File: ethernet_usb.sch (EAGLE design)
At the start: 7 parts, among them IC1 LAN9512, X1 MINI-USB_SHIELD4P-85-32004-10X

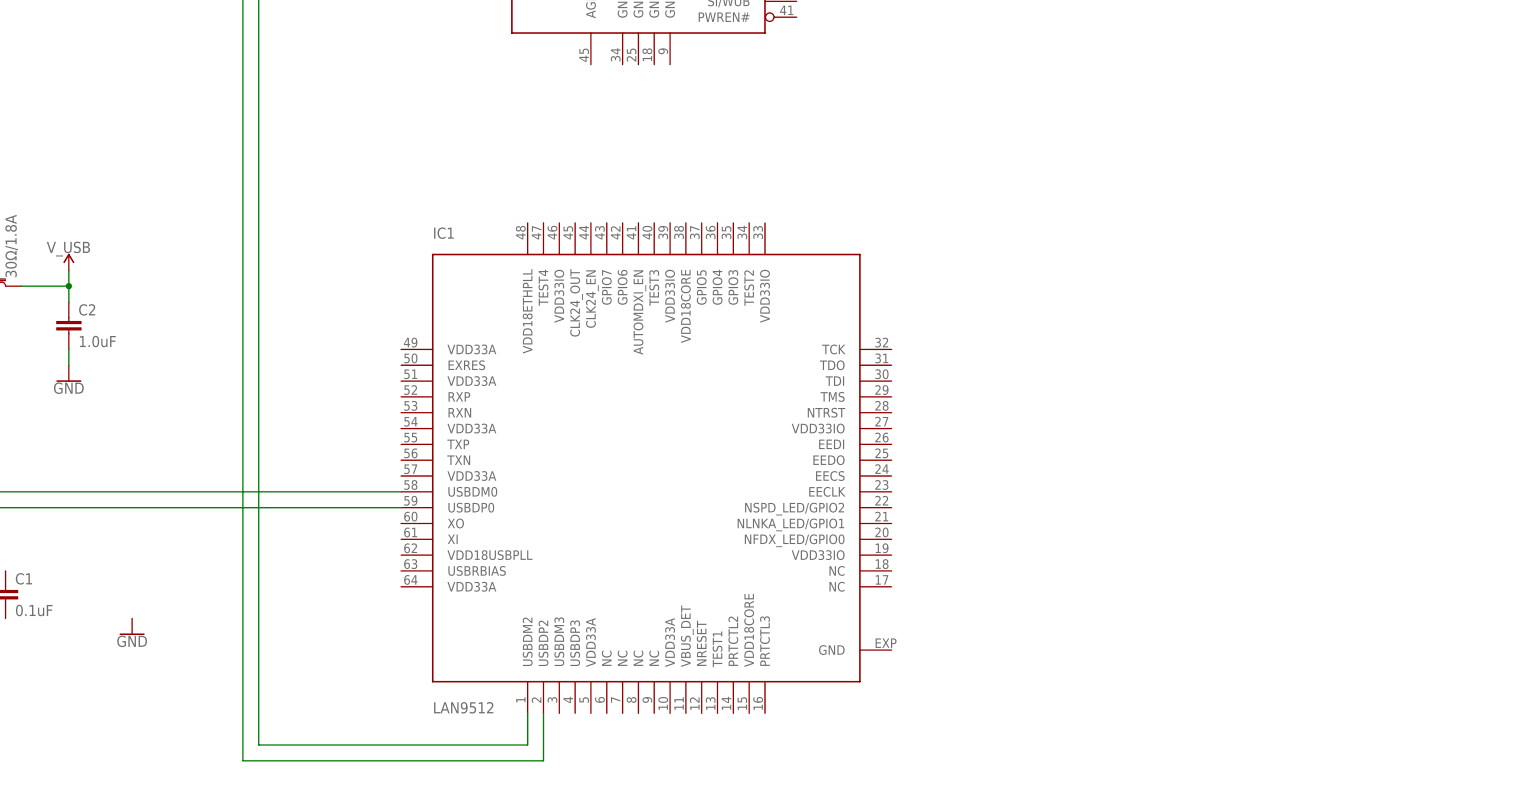
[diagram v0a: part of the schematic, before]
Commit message: snapshot
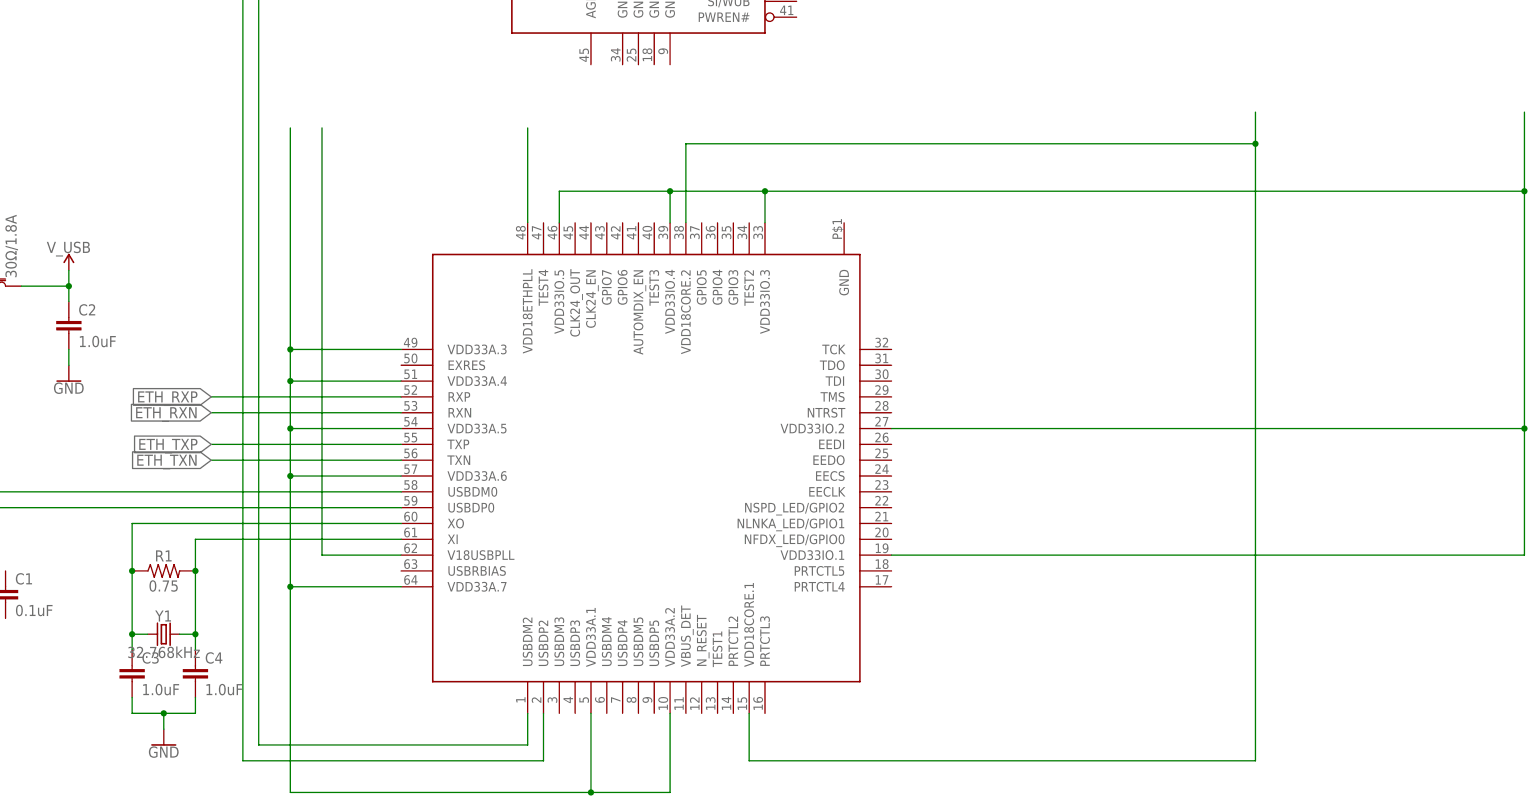
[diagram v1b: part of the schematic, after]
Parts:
- removed IC1: LAN9512, raspberrypi_cm:LAN9512
- added C3, C4: 1.0uF, SparkFun-Capacitors:1.0UF-0805-25V-10%
- added R1: 0.75, SparkFun-Resistors:0.75OHM-0805-1/4W-1%
- added U$2: LAN9514, Eagle-Library:LAN9514
- added Y1: 32.768kHz, SparkFun-Clocks:CRYSTAL-32.768KHZPTH-2X6
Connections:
- new net ETH_RXN: U$2.RXN
- new net ETH_RXP: U$2.RXP
- new net ETH_TXN: U$2.TXN
- new net ETH_TXP: U$2.TXP
- new net N$10: C3.1, R1.1, U$2.XO, Y1.1
- new net N$4: U$2.VDD18CORE.1, U$2.VDD18CORE.2
- new net N$5: U$2.VDD18ETHPLL
- new net N$6: U$2.VDD33A.1, U$2.VDD33A.2, U$2.VDD33A.3, U$2.VDD33A.4, U$2.VDD33A.5, U$2.VDD33A.6, U$2.VDD33A.7
- new net N$7: U$2.V18USBPLL
- new net N$8: U$2.VDD33IO.1, U$2.VDD33IO.2, U$2.VDD33IO.3, U$2.VDD33IO.4, U$2.VDD33IO.5
- new net N$9: C4.1, R1.2, U$2.XI, Y1.2
- net GND: now also C3.2, C4.2
- net N$1: now also U$2.USBDM2; no longer IC1.USBDM2
- net N$2: now also U$2.USBDP2; no longer IC1.USBDP2
- net USBDMHOST: now also U$2.USBDM0; no longer IC1.USBDM0
- net USBDPHOST: now also U$2.USBDP0; no longer IC1.USBDP0
